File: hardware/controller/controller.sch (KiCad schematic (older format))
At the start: 16 parts, among them J1 ADC_CONN, J2 CONN_07, J3 USB_MICRO-B_FEMALE-SMT, J4 JST_2MM_MALE, U1 MCP73831, U2 BL652

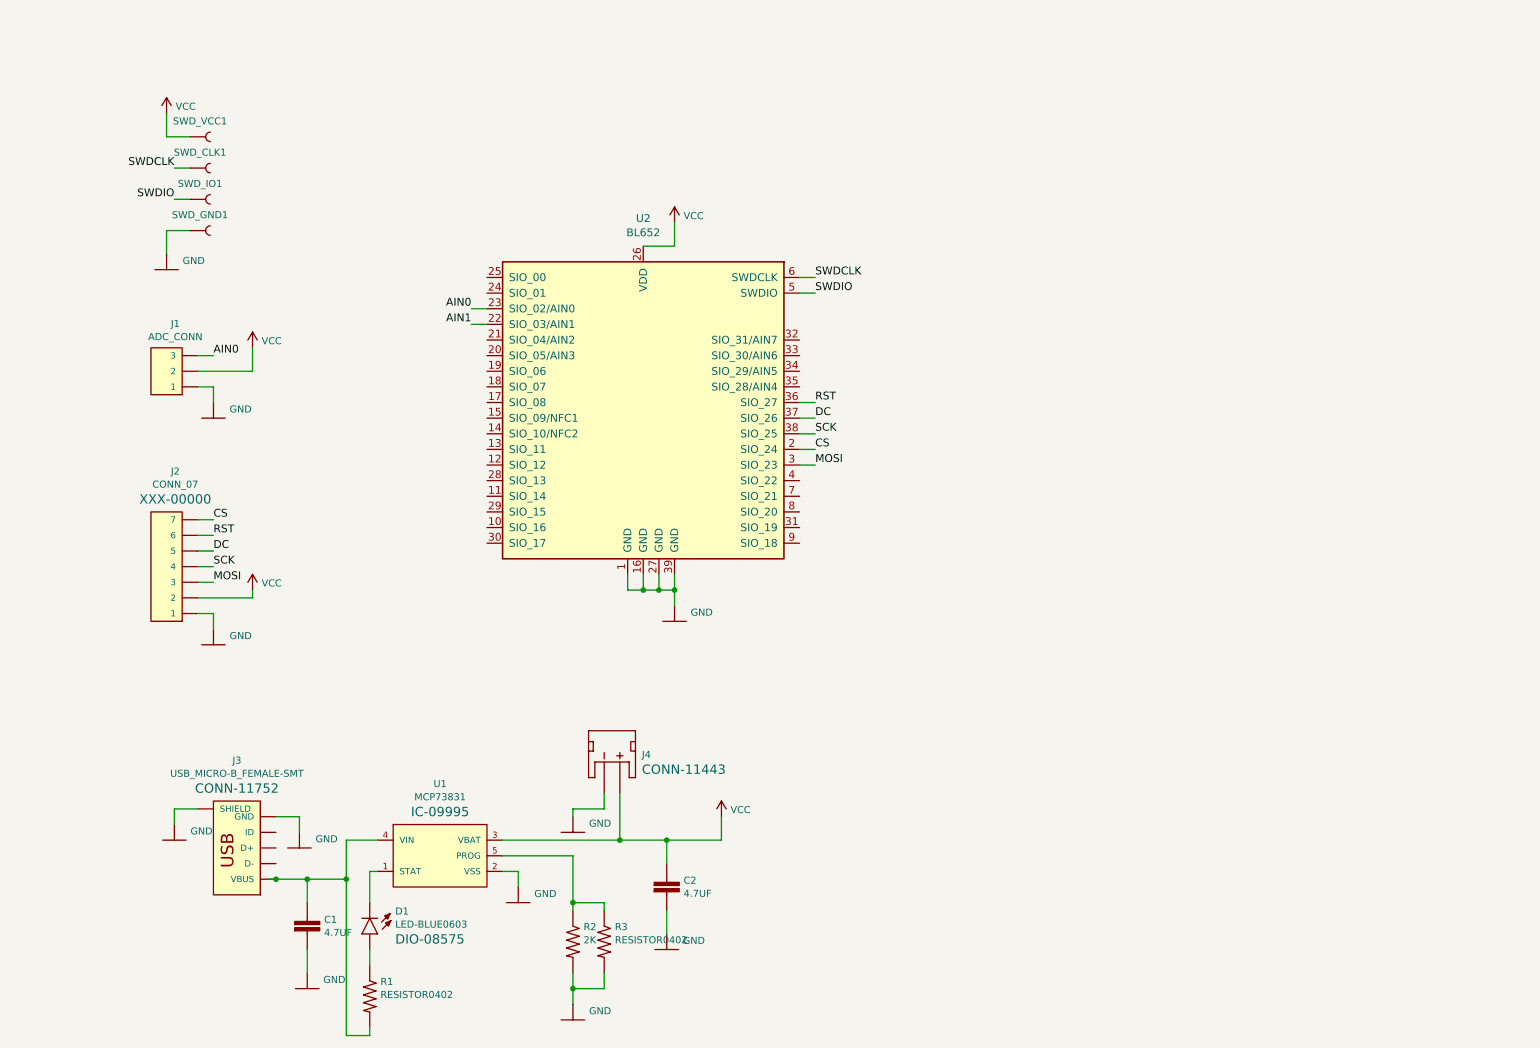
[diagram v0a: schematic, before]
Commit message: feat: finish controller pcb
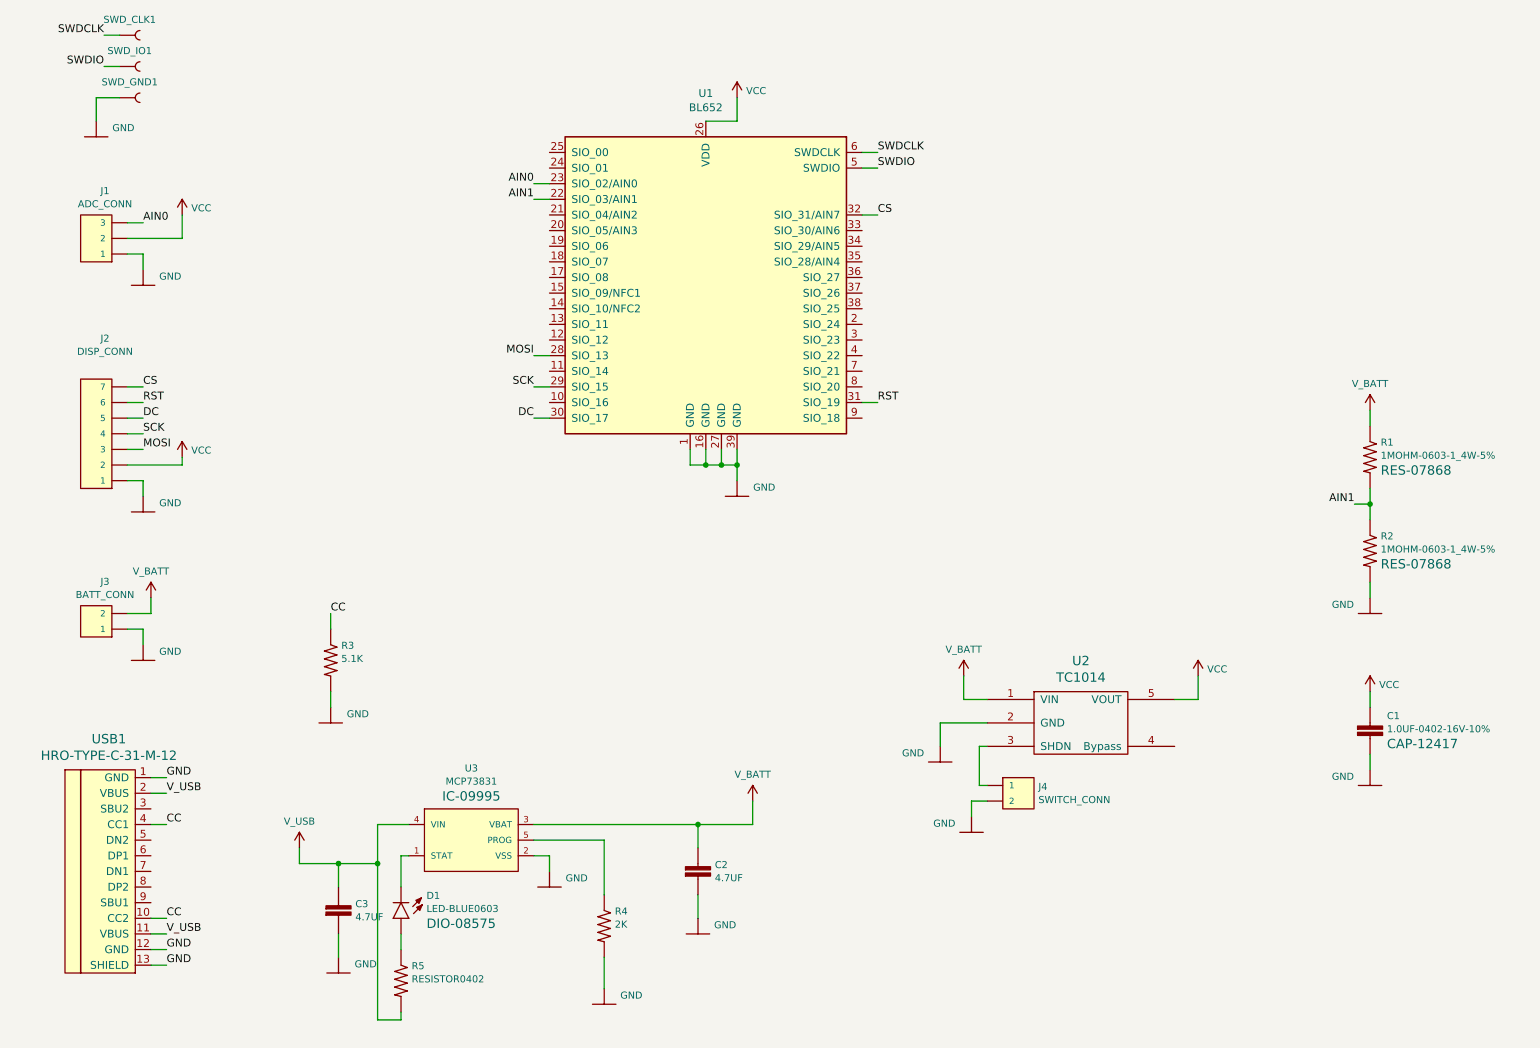
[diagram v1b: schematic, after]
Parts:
- removed J3: USB_MICRO-B_FEMALE-SMT, USB-B-MICRO-SMD, symbol SparkFun-Connectors:USB_MICRO-B_FEMALE-SMT
- removed J4: JST_2MM_MALE, JST-2-SMD, symbol SparkFun-Connectors:JST_2MM_MALE
- removed SWD_VCC1: VCC, PAD.03X.05, symbol SparkFun-Connectors:TEST-POINT3X5
- added C1: 1.0UF-0402-16V-10%, 0402, symbol SparkFun-Capacitors:1.0UF-0402-16V-10%
- added J3: BATT_CONN, 1X02, symbol SparkFun-Connectors:CONN_02
- added J4: SWITCH_CONN, 1X02, symbol SparkFun-Connectors:CONN_02
- added R1, R2: 1MOHM-0603-1_4W-5%, 0603, symbol SparkFun-Resistors:1MOHM-0603-1_4W-5%
- added U2: TC1014, Silicon-Standard:SOT23-5, symbol tinkerforge:TC1014
- added USB1: HRO-TYPE-C-31-M-12, deps:HRO-TYPE-C-31-M-12-HandSoldering, symbol Type-C:HRO-TYPE-C-31-M-12
- D1: footprint LED-0603 -> LED:LED-0603
- J1: footprint 1X03 -> Connectors:1X03
- J2: value CONN_07 -> DISP_CONN; footprint 1X07 -> Connectors:1X07; Field4 XXX-00000 -> (none)
- R3: value RESISTOR0402 -> 5.1K
- SWD_CLK1, SWD_GND1, SWD_IO1: footprint PAD.03X.05 -> Connectors:PAD.03X.05
- U3: renamed from U1; footprint SOT23-5 -> Silicon-Standard:SOT23-5
- renumbered C1 to C3, R2 to R4, R1 to R5, U2 to U1
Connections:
- net AIN1: now also R1.2, R2.1
- net CS: now also U1.32 (SIO_31/AIN7); no longer U1.2 (SIO_24)
- net DC: now also U1.30 (SIO_17); no longer U1.37 (SIO_26)
- net GND: now also C1.2, J3.1, J4.2, R2.2, U2.2 (GND), USB1.1 (GND), USB1.12 (GND), USB1.13 (SHIELD)
- net MOSI: now also U1.28 (SIO_13); no longer U1.3 (SIO_23)
- net RST: now also U1.31 (SIO_19); no longer U1.36 (SIO_27)
- net SCK: now also U1.29 (SIO_15); no longer U1.38 (SIO_25)
- net VCC: now also C1.1, U2.5 (VOUT); no longer C2.1, U3.3 (VBAT)
- net V_USB: now reaches C3.1, R5.2, U3.4 (VIN)
- net V_USB: now also USB1.11 (VBUS), USB1.2 (VBUS)
- net at R4.1, U3.5 (PROG): no longer R3.1
- new net: J4.1, U2.3 (SHDN)
- new net CC: R3.1, USB1.10 (CC2), USB1.4 (CC1)
- new net V_BATT: C2.1, J3.2, R1.1, U2.1 (VIN), U3.3 (VBAT)
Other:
- moved on the sheet: C2, C3, D1, J1, J2, R4, R5, SWD_CLK1, SWD_GND1, SWD_IO1, U1, U3
